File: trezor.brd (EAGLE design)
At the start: 50 x 26.7 mm, 27 parts, among them IC1 MCP1703CB, Q2 16MHz, U1 STM32F205RET6, U2 USB, U3 DISPLAY

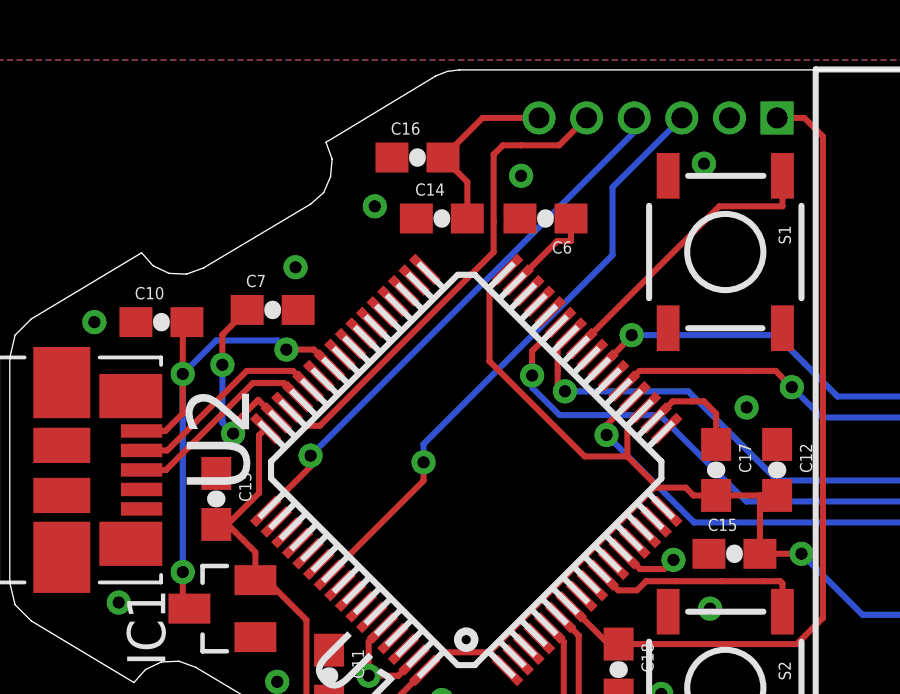
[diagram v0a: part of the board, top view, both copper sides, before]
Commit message: fix unconnected pin
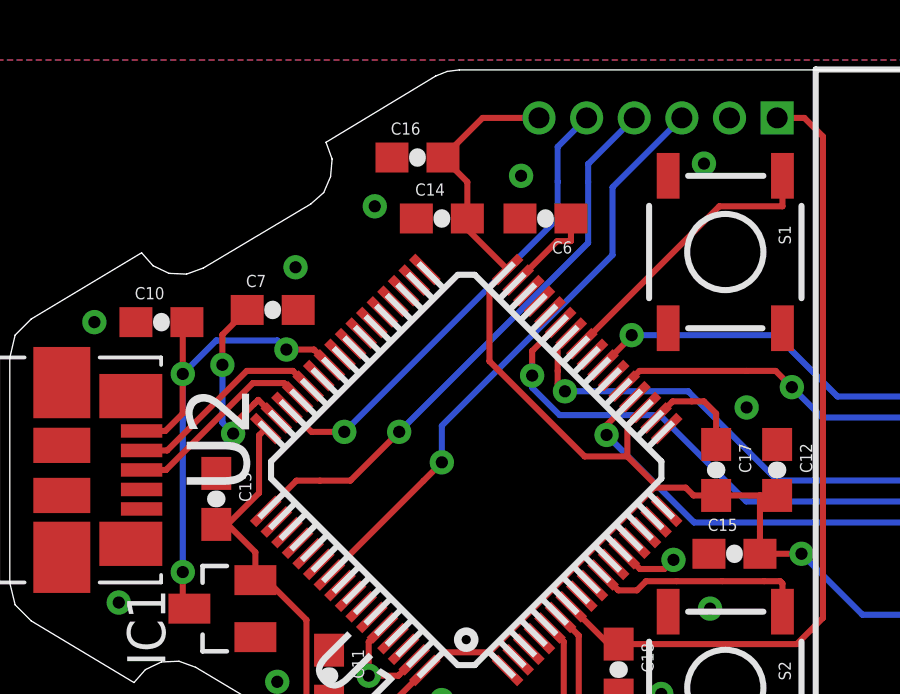
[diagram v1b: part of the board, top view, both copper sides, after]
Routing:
- net +3V3: track 86.5 -> 88.7 mm
- net N$17: track 18.2 -> 19.3 mm
- net N$15: track 16.4 -> 16.1 mm, vias 0 -> 1
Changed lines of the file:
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@@
 <wire x1="8.212" y1="10.0647" x2="9.9139" y2="8.3628" width="0.2032" layer="1"/>
 <wire x1="9.9139" y1="8.3628" x2="9.9139" y2="5.6524" width="0.2032" layer="1"/>
-<wire x1="16.6189" y1="20.0426" x2="16.0149" y2="19.4386" width="0.2032" layer="1"/>
+<wire x1="16.6189" y1="20.0426" x2="16.61885625" y2="20.04255625" width="0.2032" layer="1"/>
+<wire x1="16.61885625" y1="20.04255625" x2="16.0149" y2="19.4386" width="0.2032" layer="1"/>
 <wire x1="21.2151" y1="15.4464" x2="20.6111" y2="14.8424" width="0.2032" layer="1"/>
 <wire x1="25.0308" y1="12.5104" x2="25.6032" y2="12.5104" width="0.2032" layer="1"/>
@@
 <wire x1="40.8432" y1="8.5344" x2="28.448" y2="8.5344" width="0.2032" layer="16"/>
 <wire x1="28.448" y1="8.5344" x2="26.416" y2="10.5664" width="0.2032" layer="16"/>
+<wire x1="16.61885625" y1="20.04255625" x2="15.2772" y2="21.3842125" width="0.2032" layer="1"/>
+<wire x1="15.2772" y1="21.3842125" x2="15.2772" y2="21.7424" width="0.2032" layer="1"/>
 <wire x1="21.2151" y1="15.4464" x2="21.21505" y2="15.4463625" width="0" layer="19" extent="1-1"/>
-<wire x1="16.61885625" y1="20.04255625" x2="16.6189" y2="20.0426" width="0" layer="19" extent="1-1"/>
 <wire x1="20.861496875" y1="10.92088125" x2="20.8615" y2="10.9209" width="0" layer="19" extent="1-1"/>
 <wire x1="16.61885625" y1="6.678240625" x2="16.6189" y2="6.6782" width="0" layer="19" extent="1-1"/>
 <wire x1="8.557840625" y1="14.73925625" x2="8.5578" y2="14.7393" width="0" layer="19" extent="1-1"/>
 <wire x1="13.861140625" y1="6.678240625" x2="13.8611" y2="6.6782" width="0" layer="19" extent="1-1"/>
-<wire x1="15.2772" y1="21.7424" x2="16.6189" y2="20.0426" width="0" layer="19" extent="1-1"/>
 </signal>
 <signal name="N$1">
@@
 <wire x1="22.4282" y1="25.0952" x2="20.1168" y2="22.7838" width="0.2032" layer="16"/>
 <wire x1="20.1168" y1="22.7838" x2="20.1168" y2="20.5232" width="0.2032" layer="16"/>
-<wire x1="20.1168" y1="20.5232" x2="13.8176" y2="14.224" width="0.2032" layer="16"/>
-<wire x1="13.8176" y1="14.224" x2="13.8176" y2="13.6144" width="0.2032" layer="16"/>
 <wire x1="10.679159375" y1="9.86021875" x2="13.8176" y2="12.998659375" width="0.2032" layer="1"/>
-<wire x1="13.8176" y1="12.998659375" x2="13.8176" y2="13.6144" width="0.2032" layer="1"/>
-<via x="13.8176" y="13.6144" extent="1-16" drill="0.4064"/>
+<via x="14.4272" y="13.6144" extent="1-16" drill="0.4064"/>
+<wire x1="14.4272" y1="13.6144" x2="14.4272" y2="14.8336" width="0.2032" layer="16"/>
+<wire x1="14.4272" y1="14.8336" x2="20.1168" y2="20.5232" width="0.2032" layer="16"/>
+<wire x1="14.4272" y1="13.6144" x2="14.4272" y2="13.608259375" width="0.2032" layer="1"/>
+<wire x1="14.4272" y1="13.608259375" x2="13.8176" y2="12.998659375" width="0.2032" layer="1"/>
 </signal>
 <signal name="N$15">
 <contactref element="U1" pad="46"/>
 <contactref element="U$2" pad="5"/>
-<wire x1="9.264946875" y1="15.4463625" x2="9.877709375" y2="14.8336" width="0.2032" layer="1"/>
-<wire x1="9.877709375" y1="14.8336" x2="10.3632" y2="14.8336" width="0.2032" layer="1"/>
-<wire x1="10.3632" y1="14.8336" x2="16.1544" y2="20.6248" width="0.2032" layer="1"/>
-<wire x1="16.1544" y1="20.6248" x2="16.1544" y2="21.6408" width="0.2032" layer="1"/>
-<wire x1="19.2532" y1="25.0952" x2="18.3388" y2="24.1808" width="0.2032" layer="1"/>
-<wire x1="18.3388" y1="24.1808" x2="17.0688" y2="24.1808" width="0.2032" layer="1"/>
-<wire x1="17.0688" y1="24.1808" x2="16.4592" y2="24.1808" width="0.2032" layer="1"/>
-<wire x1="16.4592" y1="24.1808" x2="16.1544" y2="23.876" width="0.2032" layer="1"/>
-<wire x1="16.1544" y1="23.876" x2="16.1544" y2="21.6408" width="0.2032" layer="1"/>
+<wire x1="9.264946875" y1="15.4463625" x2="10.080909375" y2="14.6304" width="0.2032" layer="1"/>
+<wire x1="10.080909375" y1="14.6304" x2="11.176" y2="14.6304" width="0.2032" layer="1"/>
+<via x="11.176" y="14.6304" extent="1-16" drill="0.4064"/>
+<wire x1="11.176" y1="14.6304" x2="18.288" y2="21.7424" width="0.2032" layer="16"/>
+<wire x1="18.288" y1="21.7424" x2="18.288" y2="22.9616" width="0.2032" layer="16"/>
+<wire x1="18.288" y1="22.9616" x2="18.288" y2="24.13" width="0.2032" layer="16"/>
+<wire x1="18.288" y1="24.13" x2="19.2532" y2="25.0952" width="0.2032" layer="16"/>
 </signal>
 <signal name="N$17">
 <contactref element="U1" pad="49"/>
-<wire x1="10.053" y1="13.8368" x2="17.6657" y2="21.4495" width="0.2032" layer="16"/>
-<via x="10.053" y="13.8368" extent="1-16" drill="0.4064" diameter="0.8128"/>
-<wire x1="8.557840625" y1="11.981540625" x2="10.053" y2="13.4767" width="0.2032" layer="1"/>
-<wire x1="10.053" y1="13.4767" x2="10.053" y2="13.8368" width="0.2032" layer="1"/>
 <contactref element="U$2" pad="4"/>
-<wire x1="17.6657" y1="21.4495" x2="20.8407" y2="24.6245" width="0.2032" layer="16"/>
-<wire x1="20.8407" y1="24.6245" x2="20.8407" y2="25.0952" width="0.2032" layer="16"/>
+<via x="13.0048" y="14.6304" extent="1-16" drill="0.4064"/>
+<wire x1="13.0048" y1="14.6304" x2="19.304" y2="20.9296" width="0.2032" layer="16"/>
+<wire x1="19.304" y1="20.9296" x2="19.304" y2="22.9616" width="0.2032" layer="16"/>
+<wire x1="19.304" y1="22.9616" x2="19.304" y2="23.5585" width="0.2032" layer="16"/>
+<wire x1="19.304" y1="23.5585" x2="20.8407" y2="25.0952" width="0.2032" layer="16"/>
+<wire x1="8.557840625" y1="11.981540625" x2="9.5811" y2="13.0048" width="0.2032" layer="1"/>
+<wire x1="9.5811" y1="13.0048" x2="10.3632" y2="13.0048" width="0.2032" layer="1"/>
+<wire x1="10.3632" y1="13.0048" x2="11.3792" y2="13.0048" width="0.2032" layer="1"/>
+<wire x1="11.3792" y1="13.0048" x2="13.0048" y2="14.6304" width="0.2032" layer="1"/>
 </signal>
 <signal name="N$19">

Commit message: change crystal
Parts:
- Q2: value 16MHz -> 8MHz
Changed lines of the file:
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@@
 <element name="S1" library="SparkFun-Electromechanical" package="TACTILE_SWITCH_SMD" value="SWITCH-MOMENTARY-2SMD" x="23.876" y="20.6248" rot="R270"/>
 <element name="S2" library="SparkFun-Electromechanical" package="TACTILE_SWITCH_SMD" value="SWITCH-MOMENTARY-2SMD" x="23.876" y="6.096" rot="R270"/>
-<element name="Q2" library="crystal" package="CTS406" value="16MHz" x="17.6784" y="2.8448" rot="R180"/>
+<element name="Q2" library="crystal" package="CTS406" value="8MHz" x="17.6784" y="2.8448" rot="R180"/>
 <element name="C9" library="SparkFun-Passives" package="0603-CAP" value="22pF" x="23.1648" y="1.4224"/>
 <element name="C8" library="SparkFun-Passives" package="0603-CAP" value="22pF" x="13.0048" y="3.6576" rot="R90"/>
